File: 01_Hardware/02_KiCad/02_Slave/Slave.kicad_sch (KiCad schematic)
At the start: 12 parts, among them J1 Screw_Terminal_01x04, J2 Conn_01x30_Female, J3 Screw_Terminal_01x04, J4 Conn_01x30_Female, Q1 AO3400A, Q2 AO3400A, U1 LM393

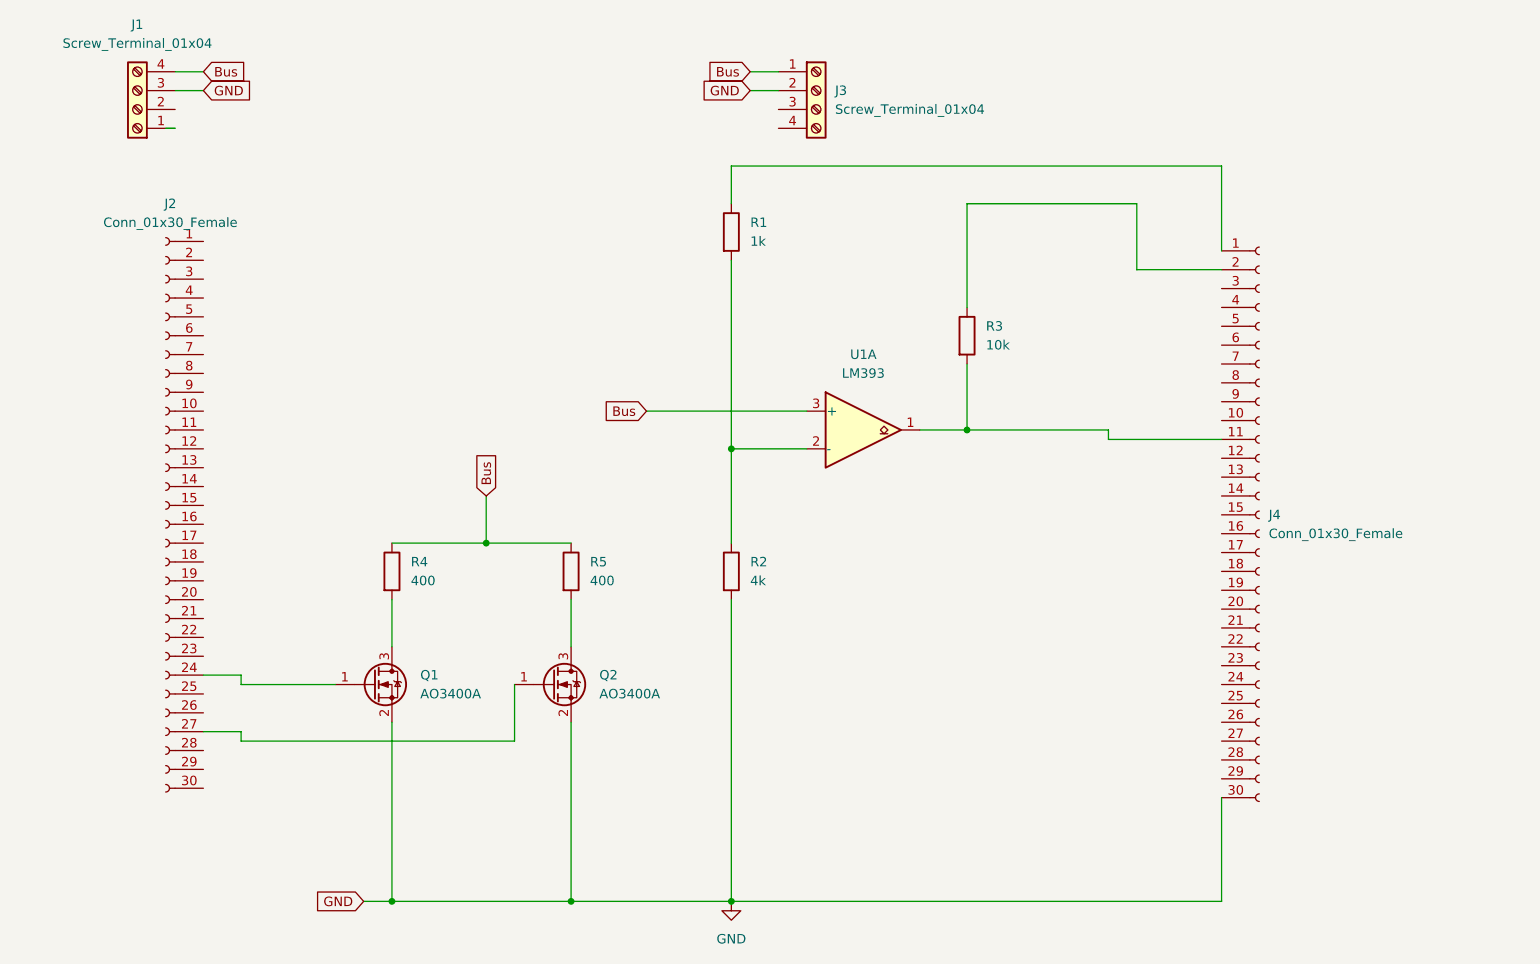
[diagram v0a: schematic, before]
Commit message: KiCAD
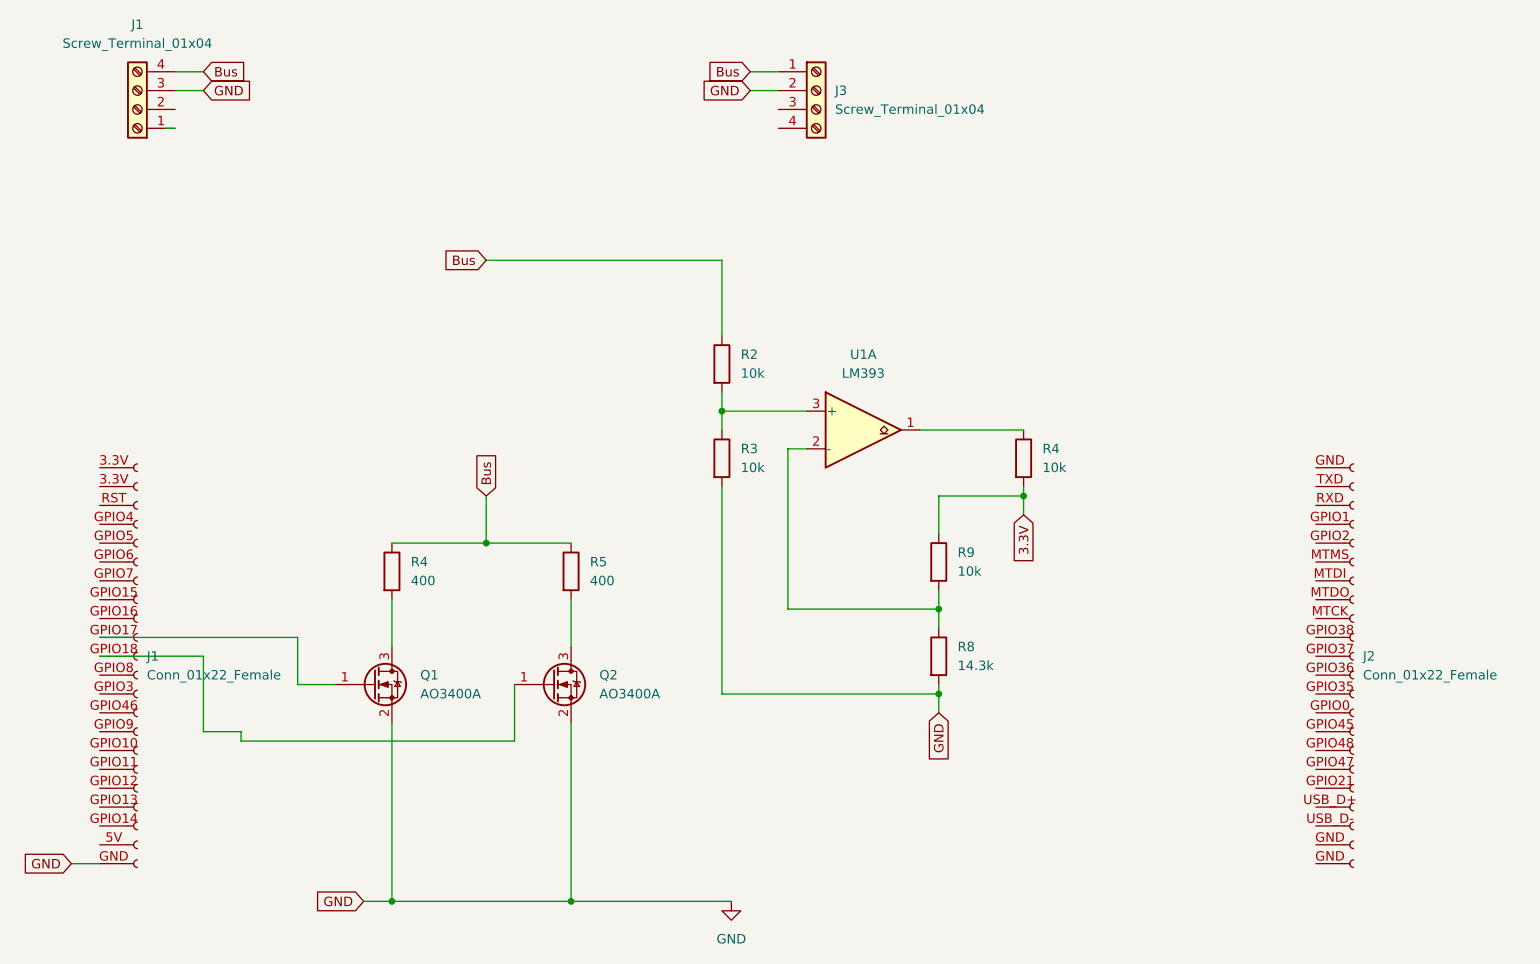
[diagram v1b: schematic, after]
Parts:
- removed J2, J4: Conn_01x30_Female, Connector_PinSocket_2.54mm:PinSocket_1x30_P2.54mm_Vertical, symbol Connector:Conn_01x30_Female
- removed R1: 1k, Resistor_THT:R_Axial_DIN0204_L3.6mm_D1.6mm_P5.08mm_Horizontal, symbol Device:R
- added J1, J2: Conn_01x22_Female, symbol Connector:Conn_01x22_Female
- added R4, R9: 10k, symbol Device:R
- added R8: 14.3k, symbol Device:R
- R2: value 4k -> 10k; footprint Resistor_THT:R_Axial_DIN0204_L3.6mm_D1.6mm_P5.08mm_Horizontal -> (none)
- R3: footprint Resistor_THT:R_Axial_DIN0204_L3.6mm_D1.6mm_P5.08mm_Horizontal -> (none)
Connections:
- net Bus: now also R2.1; no longer U1.3 (+)
- net GND: now also R3.2, J1.GND (Pin_22), R8.2; no longer R2.2
- net at Q1.1 (G): now also J1.GPIO17 (Pin_10)
- net at Q2.1 (G): now also J1.GPIO18 (Pin_11)
- net at U1.2 (-): now also R8.1, R9.2; no longer R2.1
- net at U1.1: now also R4.1; no longer R3.2
- net at R3.1: now also R2.2, U1.3 (+)
- new net 3.3V: R4.2, R9.1
